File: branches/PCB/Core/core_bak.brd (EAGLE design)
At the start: 51.7 x 73.7 mm, 21 parts, among them U1 PIC32MX230F064B-

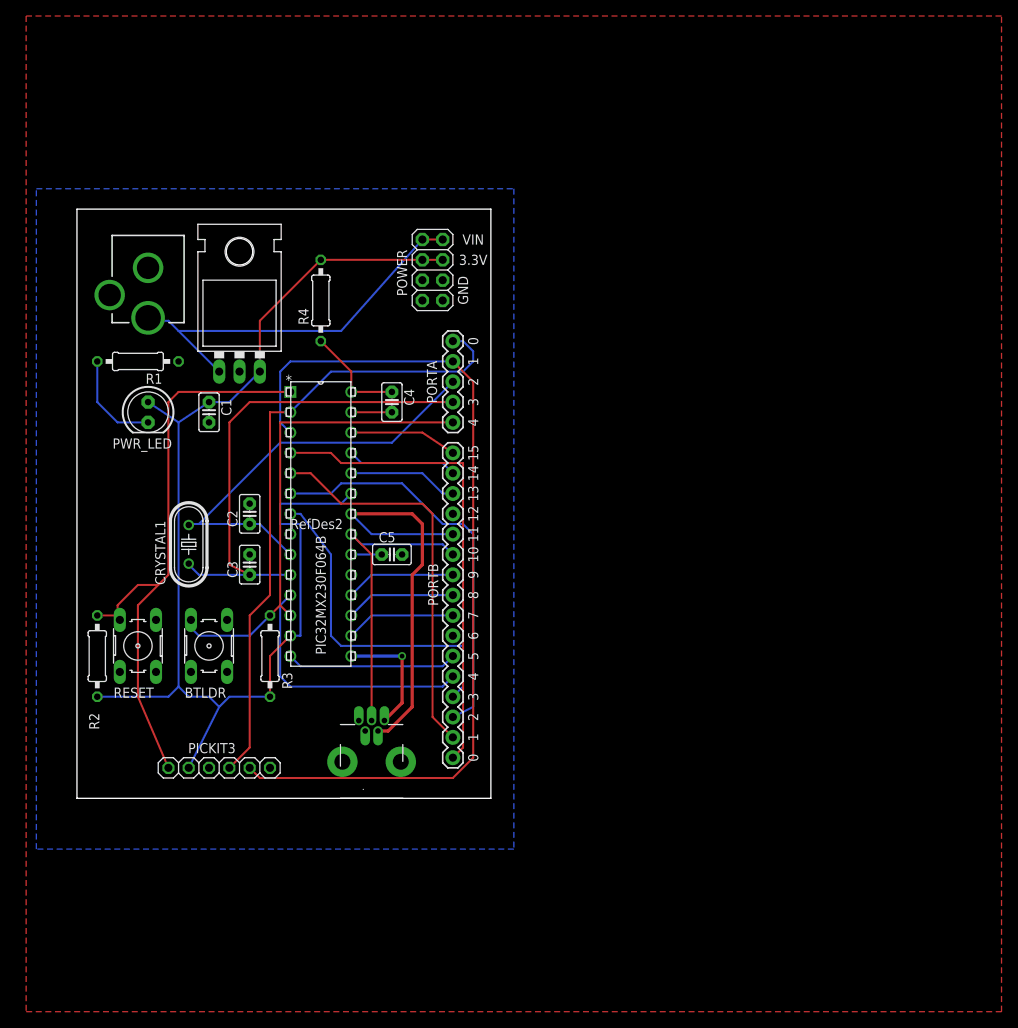
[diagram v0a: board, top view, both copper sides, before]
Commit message: Pre Gerber for Rev 1.00
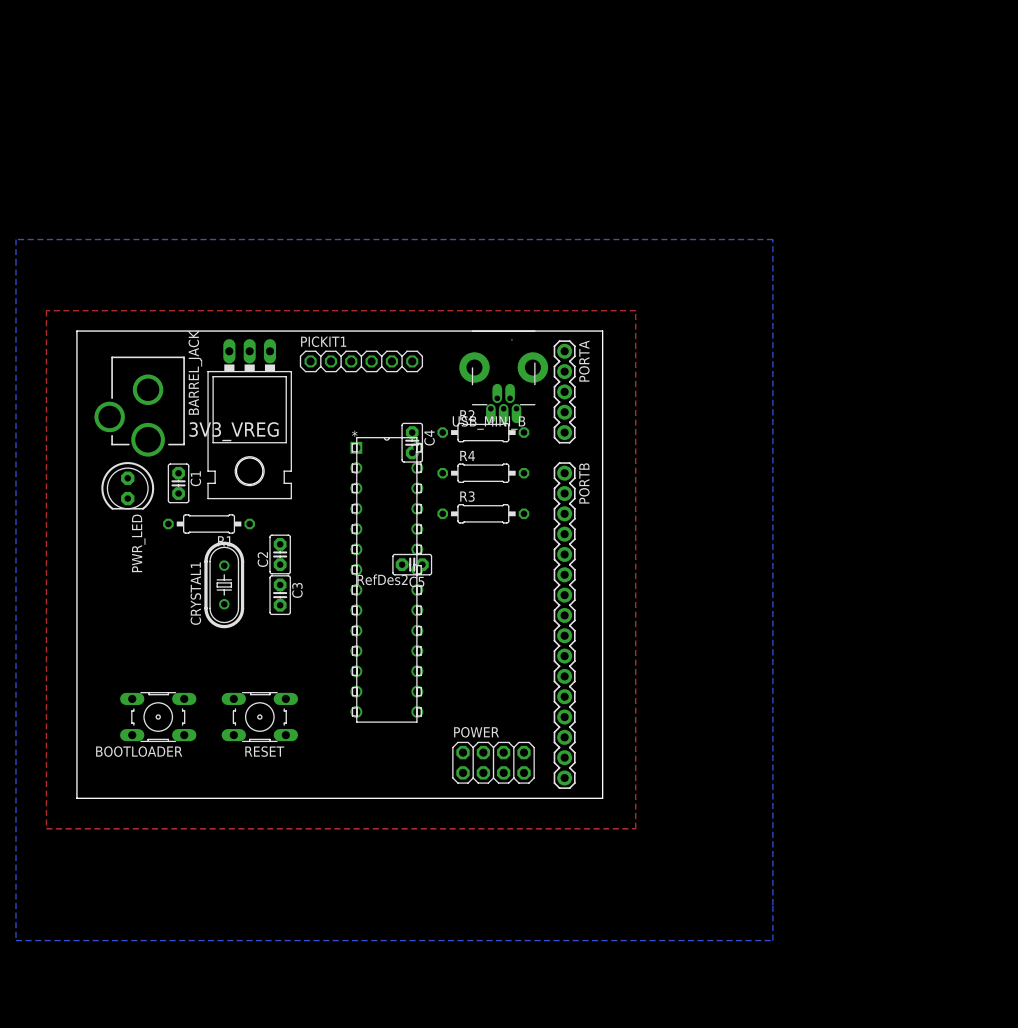
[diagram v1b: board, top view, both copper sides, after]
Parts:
- removed BTLDR: (no value), switch-omron:B3F-10XX
- removed PICKIT3: (no value), adafruit:1X06
- added BOOTLOADER: (no value), switch-omron:B3F-10XX
- added PICKIT1: (no value), adafruit:1X06
- moved POWER 62.1 mm to (52.1, 4.45), turned to 0 degrees
- moved USB_MINI_B 60.7 mm to (53.3, 58.4), turned to 180 degrees
- moved R2 55.8 mm to (50.8, 45.7), turned to 0 degrees
- moved PORTB 38.2 mm to (61.0, 40.6), turned to 270 degrees
- moved R3 32.1 mm to (50.8, 35.6), turned to 0 degrees
- moved R4 29.6 mm to (50.8, 40.6), turned to 0 degrees
- moved R1 22.2 mm to (16.5, 34.3)
- moved RESET 17.6 mm to (22.9, 10.2), turned to 180 degrees
- moved BARREL_JACK 15.2 mm to (8.89, 58.4)
- moved PORTA 14.0 mm to (61.0, 55.9)
- moved U1 10.8 mm to (42.5, 10.8)
- moved PWR_LED 9.86 mm to (6.35, 38.7)
- moved C1 9.67 mm to (12.7, 39.4)
- moved CRYSTAL1 6.75 mm to (18.4, 26.7)
- moved C2 6.35 mm to (25.4, 30.5)
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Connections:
- net +3V3: now also PICKIT1.2; no longer PICKIT3.2
- net D-: now also USB_MINI_B.D-; no longer USB_MINI_B.ID
- net GND: now also BOOTLOADER.1, PICKIT1.3, USB_MINI_B.GND; no longer BTLDR.1, PICKIT3.3, USB_MINI_B.VBUS
- net MCLR: now also PICKIT1.1; no longer PICKIT3.1
- net RA0: now also PICKIT1.4, PICKIT1.5, PICKIT1.6; no longer PICKIT3.4
- net RA1: no longer PICKIT3.5
- net RA4: now also BOOTLOADER.3; no longer BTLDR.3
- net VBUS: now also USB_MINI_B.VBUS; no longer USB_MINI_B.GND
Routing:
- net +3V3: track 153.1 -> 0.00 mm
- net RA1: track 110.4 -> 0.00 mm
- net RA0: track 78.9 -> 0.00 mm
- net MCLR: track 74.4 -> 0.00 mm
- net OSC2: track 63.0 -> 0.00 mm
- net RA4: track 60.5 -> 0.00 mm
- net RB0: track 59.5 -> 0.00 mm
- net OSC1: track 53.5 -> 0.00 mm
- net D-: track 52.1 -> 0.00 mm
- net RB2: track 50.4 -> 0.00 mm
- net +5V: track 49.7 -> 0.00 mm
- net RB1: track 48.9 -> 0.00 mm
- net RB3: track 41.7 -> 0.00 mm
- net D+: track 38.1 -> 0.00 mm
- net RB4: track 33.3 -> 0.00 mm
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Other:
- board size 51.7 x 73.7 mm -> 65.7 x 58.4 mm
- board text removed: "0"
- board text removed: "1"
- board text removed: "10"
- board text removed: "11"
- board text removed: "12"
- board text removed: "13"
- board text removed: "14"
- board text removed: "15"
- board text removed: "2"
- board text removed: "3"
- board text removed: "3.3V"
- board text removed: "4"
- board text removed: "5"
- board text removed: "6"
- board text removed: "7"
- board text removed: "8"
- board text removed: "9"
- board text removed: "GND"
- board text removed: "PIC32MX230F064B"
- board text removed: "VIN"
